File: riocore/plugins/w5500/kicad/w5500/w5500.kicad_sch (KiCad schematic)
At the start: 34 parts, among them J6 RJ45_Pulse_J0011D21BNL, U8 W5500, Y2 Crystal_25MHz

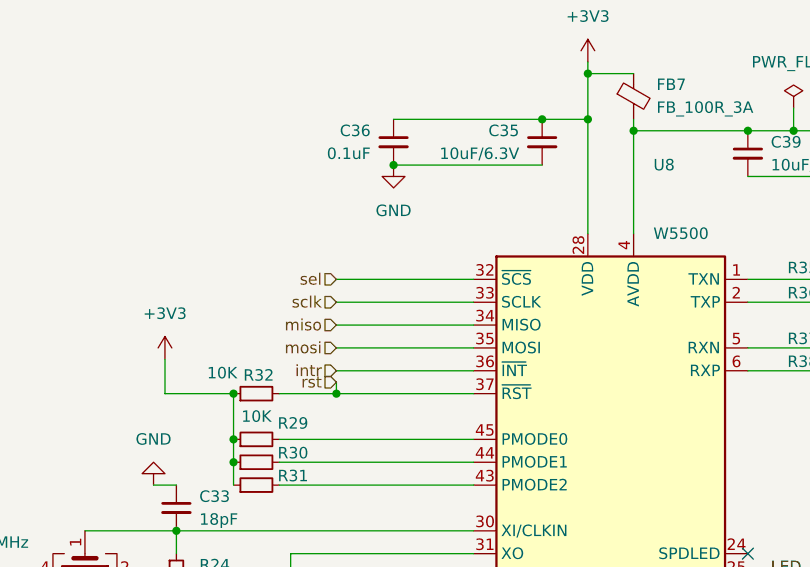
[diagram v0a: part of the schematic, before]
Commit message: some changes
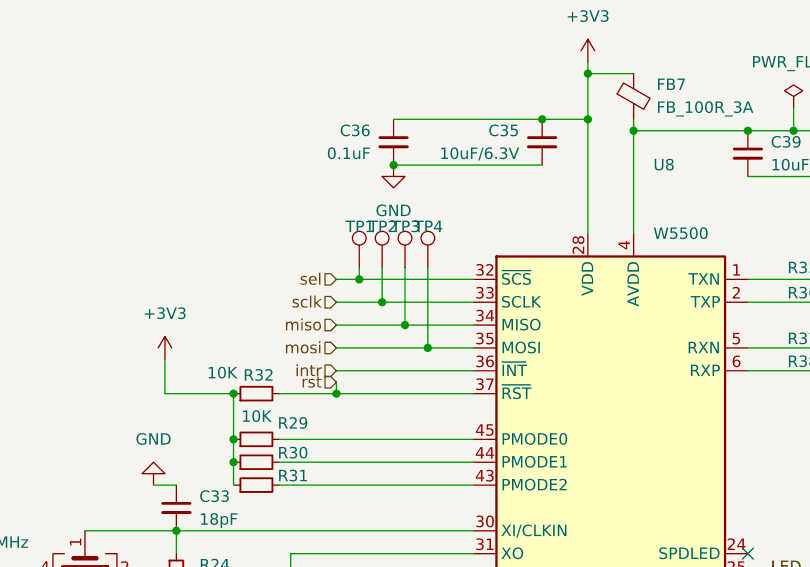
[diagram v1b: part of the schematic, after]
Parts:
- added TP1, TP2, TP3, TP4: TestPoint, TestPoint:TestPoint_Pad_D1.0mm, symbol Connector:TestPoint
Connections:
- net miso: now also TP3.1
- net mosi: now also TP4.1
- net sclk: now also TP2.1
- net sel: now also TP1.1
